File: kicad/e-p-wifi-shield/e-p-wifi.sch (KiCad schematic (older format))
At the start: 32 parts, among them J1 Shunt, J2 Vbat1, J3 Masse T1, J4 Température, J5 Vbat2, J6 Conn_02x14_MKR1010, SW1 StSp - Farnell 986-501, SW2 Sleep - Farnell 986-501, SW3 Conrad 711771

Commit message: Ajout du logo A3C
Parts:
- J4: footprint Connector_PinHeader_1.00mm:PinHeader_1x06_P1.00mm_Vertical -> Connector_PinHeader_2.54mm:PinHeader_1x06_P2.54mm_Vertical
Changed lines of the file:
@@
 F 0 "J4" H 3013 2998 50  0000 C CNN
 F 1 "Température" H 2867 2655 50  0000 C CNN
-F 2 "Connector_PinHeader_1.00mm:PinHeader_1x06_P1.00mm_Vertical" H 2851 3050 50  0001 C CNN
+F 2 "Connector_PinHeader_2.54mm:PinHeader_1x06_P2.54mm_Vertical" H 2851 3050 50  0001 C CNN
 F 3 "~" H 2851 3050 50  0001 C CNN
 	1    2851 3050

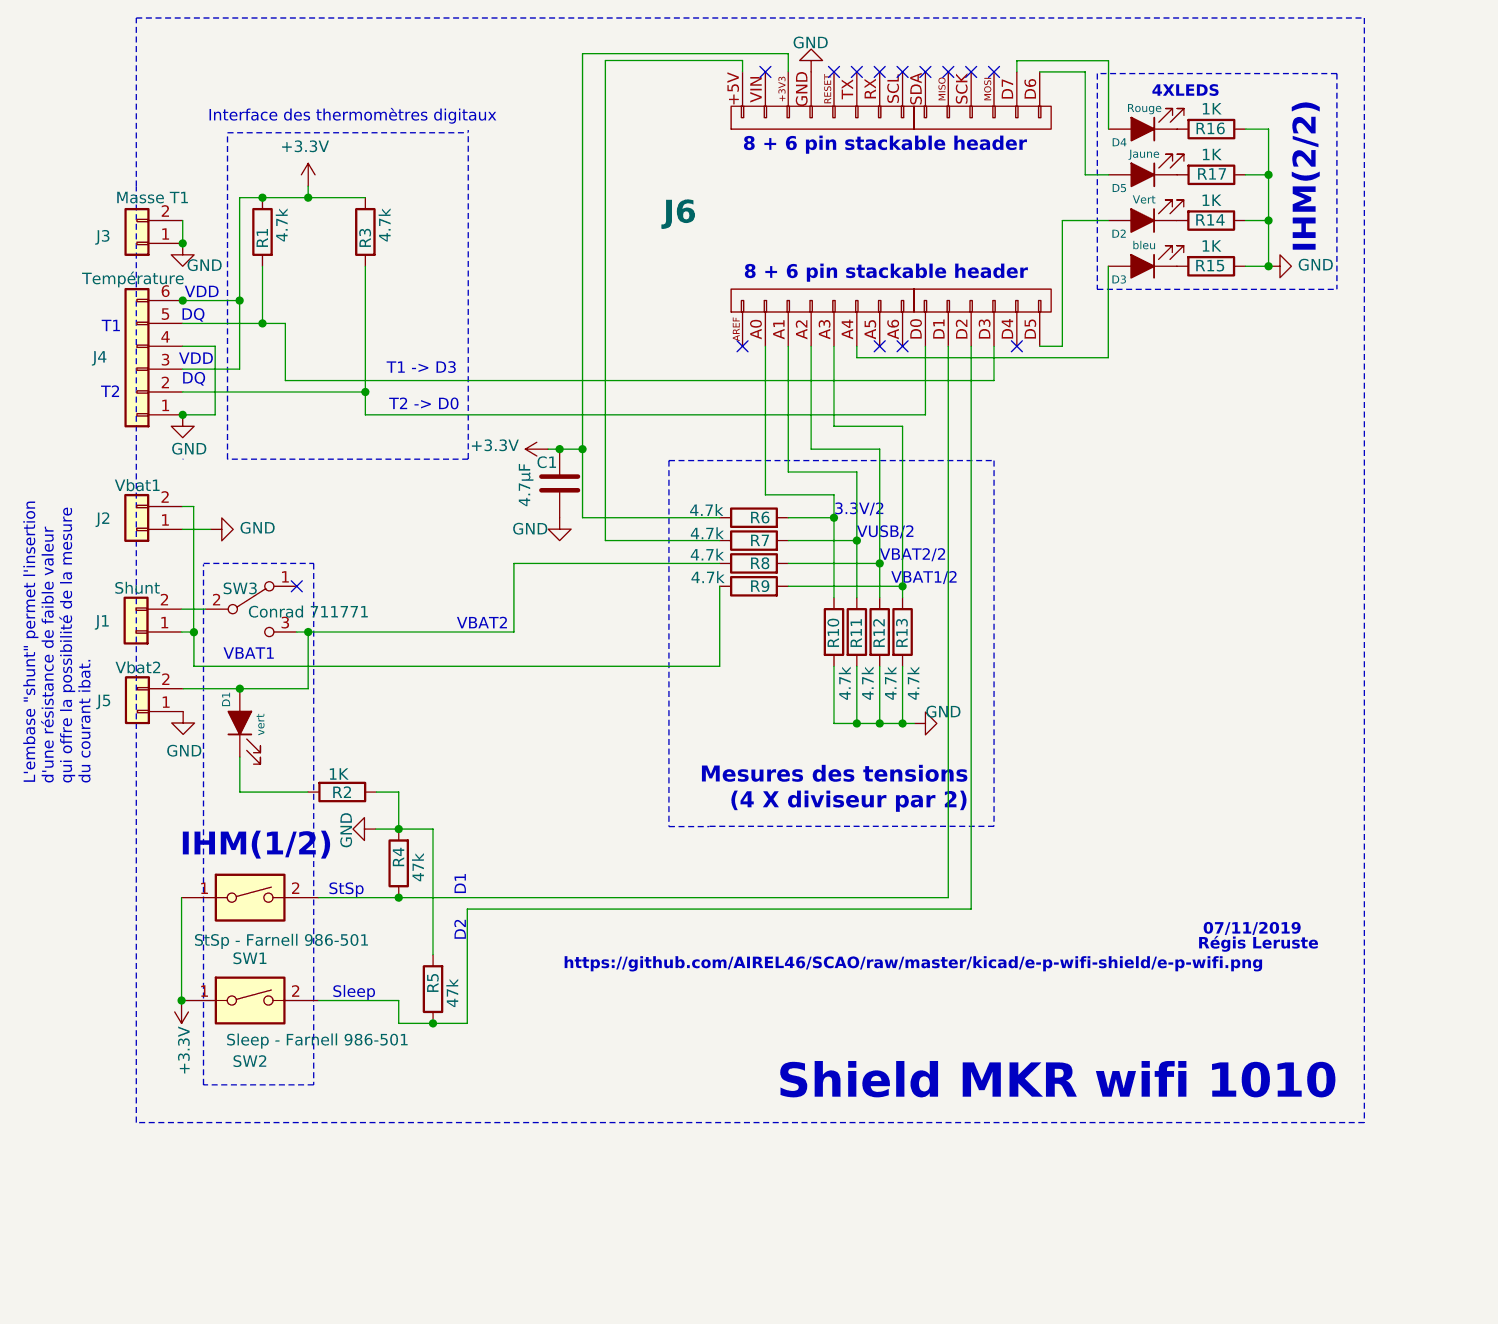
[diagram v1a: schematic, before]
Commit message: Maj du 20/11/2019
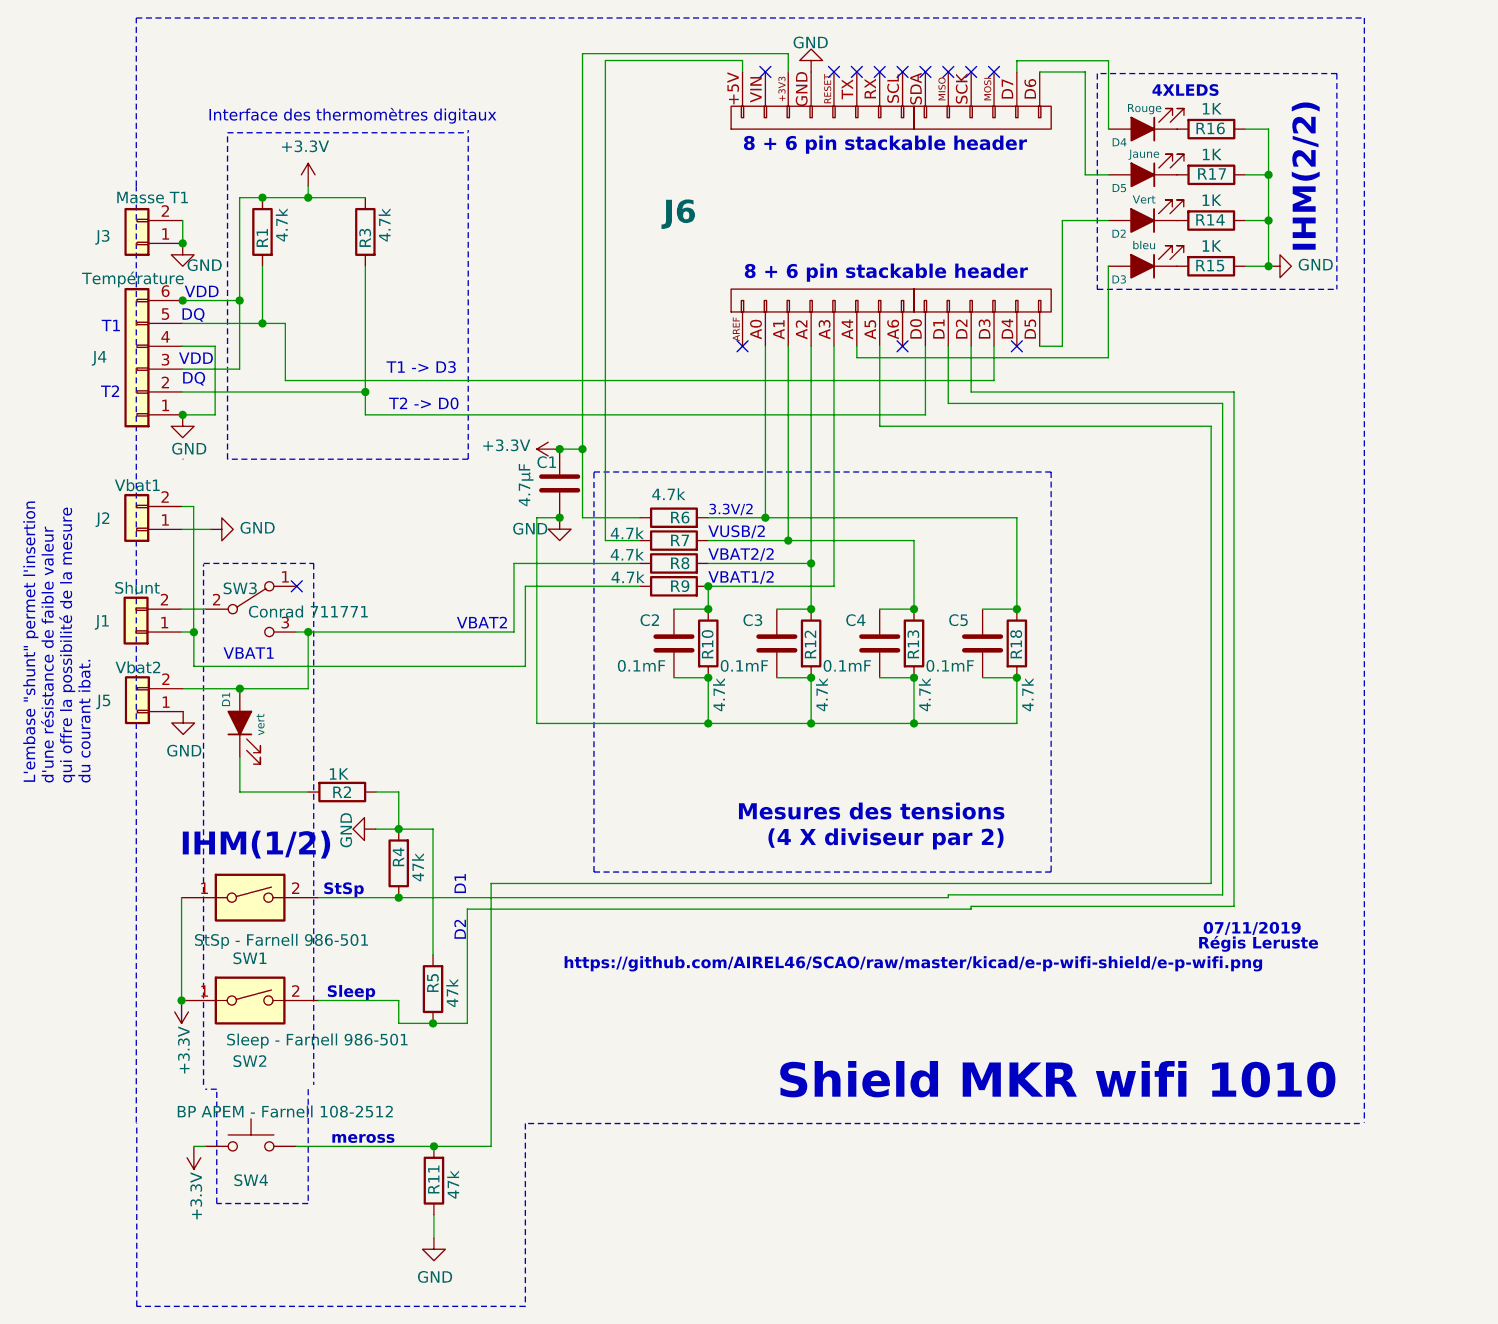
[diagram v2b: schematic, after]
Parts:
- added C2, C3, C4, C5: 0.1mF, Capacitor_THT:C_Disc_D3.0mm_W1.6mm_P2.50mm, symbol Device:C
- added R18: 4.7k, Resistor_THT:R_Axial_DIN0207_L6.3mm_D2.5mm_P7.62mm_Horizontal, symbol Device:R
- added SW4: BP APEM - Farnell 108-2512, MKR1010:BP, symbol Switch:SW_Push
- R11: value 4.7k -> 47k
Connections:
- net +3V3: now also SW4.1
- net GND: now also R11.1, C2.2, C3.2, C4.2, C5.2, R18.2; no longer R11.2
- net at J6.A0 (Pin_2), R6.2: now also C5.1, R18.1; no longer R10.1
- net at J6.A1 (Pin_3), R7.2: now also R13.1, C4.1; no longer R11.1
- net at J6.A2 (Pin_4), R12.1, R8.2: now also C3.1
- net at J6.A3 (Pin_5), R9.2: now also R10.1, C2.1; no longer R13.1
- net at J6.A5 (Pin_7): now also R11.2, SW4.2
- no-connect marks 14 -> 13
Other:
- note added: "meross"
- moved on the sheet: R10, R6, R7, R8, R9

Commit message: Copie des fichiers kicad de Mikaël
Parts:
- J6: footprint MKR1010:PinSocket_2x14_MKR1010 -> e-p-wifi-v2:PinSocket_2x14_MKR1010
- SW1, SW2: footprint MKR1010:jumper-switch -> e-p-wifi-v2:jumper-switch
- SW3: footprint MKR1010:switch -> e-p-wifi-v2:switch
- SW4: footprint MKR1010:BP -> e-p-wifi-v2:BP
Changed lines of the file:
@@
 F 0 "SW3" H 3303 4189 50  0000 C CNN
 F 1 "Conrad 711771" H 3602 4087 50  0000 C CNN
-F 2 "MKR1010:switch" H 3350 4100 50  0001 C CNN
+F 2 "e-p-wifi-v2:switch" H 3350 4100 50  0001 C CNN
 F 3 "https://produktinfo.conrad.com/datenblaetter/700000-724999/711771-da-01-en-MINI_SCHIEBESCHALTER_450302014072.PDF" H 3350 4100 50  0001 C CNN
 	1    3350 4100
@@
 F 0 "SW1" H 3346 5095 50  0000 C CNN
 F 1 "StSp - Farnell 986-501" H 3484 5175 50  0000 C CNN
-F 2 "MKR1010:jumper-switch" H 3346 5362 50  0001 C CNN
+F 2 "e-p-wifi-v2:jumper-switch" H 3346 5362 50  0001 C CNN
 F 3 "http://www.farnell.com/datasheets/58539.pdf?_ga=2.27608380.140208918.1573048803-1966718086.1557591461&_gac=1.121467258.1573048803.Cj0KCQiA-4nuBRCnARIsAHwyuPqR51EVzwLC_rjGxuRlpl_aeelUyUlwni0GneFg4tO4wrwk64y3RFoaAuRiEALw_wcB" H 3346 5362 50  0001 C CNN
 	1    3346 5362
@@
 F 0 "SW2" H 3346 5545 50  0000 C CNN
 F 1 "Sleep - Farnell 986-501" H 3641 5639 50  0000 C CNN
-F 2 "MKR1010:jumper-switch" H 3346 5812 50  0001 C CNN
+F 2 "e-p-wifi-v2:jumper-switch" H 3346 5812 50  0001 C CNN
 F 3 "http://www.farnell.com/datasheets/58539.pdf?_ga=2.27608380.140208918.1573048803-1966718086.1557591461&_gac=1.121467258.1573048803.Cj0KCQiA-4nuBRCnARIsAHwyuPqR51EVzwLC_rjGxuRlpl_aeelUyUlwni0GneFg4tO4wrwk64y3RFoaAuRiEALw_wcB" H 3346 5812 50  0001 C CNN
 	1    3346 5812
@@
 F 0 "J6" V 6487 3697 100 0000 R CNB
 F 1 "Conn_02x14_MKR1010" V 6479 3339 75  0001 R CNB
-F 2 "MKR1010:PinSocket_2x14_MKR1010" V 6249 2680 50  0001 C CNN
+F 2 "e-p-wifi-v2:PinSocket_2x14_MKR1010" V 6249 2680 50  0001 C CNN
 F 3 "~" H 6100 2750 50  0001 C CNN
 	1    6100 2750
@@
 F 0 "SW4" H 3350 6300 50  0000 C CNN
 F 1 "BP APEM - Farnell 108-2512" H 3500 6600 50  0000 C CNN
-F 2 "MKR1010:BP" H 3350 6650 50  0001 C CNN
+F 2 "e-p-wifi-v2:BP" H 3350 6650 50  0001 C CNN
 F 3 "http://www.farnell.com/datasheets/10672.pdf?_ga=1.98306207.1823820493.1466675868" H 3350 6650 50  0001 C CNN
 	1    3350 6450
